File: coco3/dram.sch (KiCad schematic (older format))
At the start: 3 parts, among them CN4 Conn_01x12_Female, CN5 Conn_01x12_Female, CN6 Conn_01x12_Female

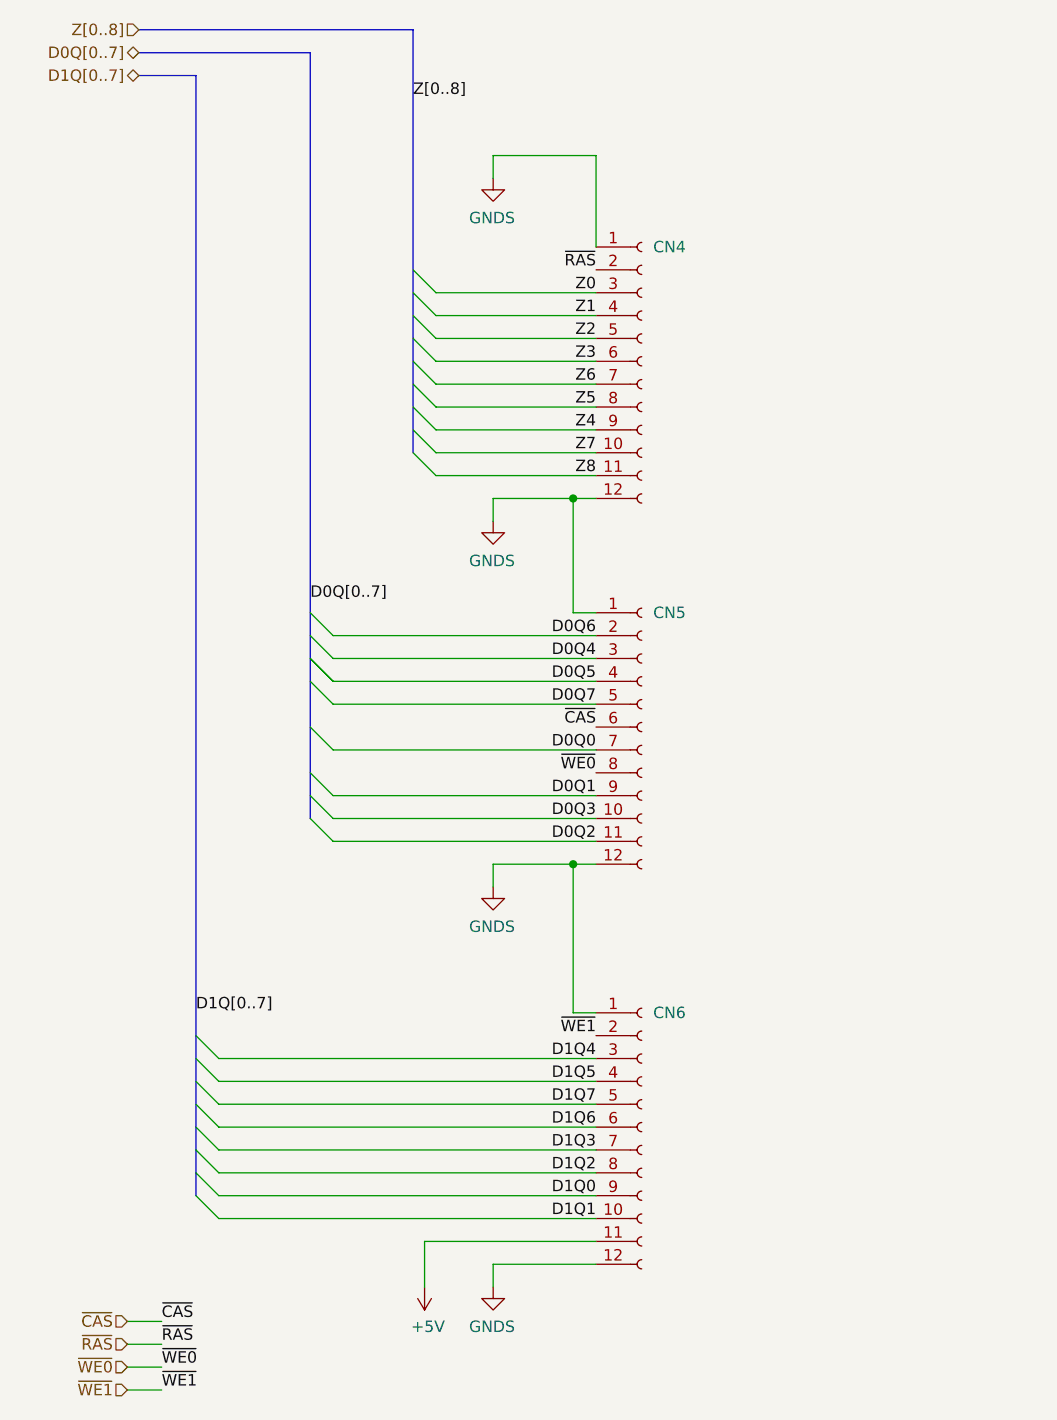
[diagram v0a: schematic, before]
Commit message: routed the board
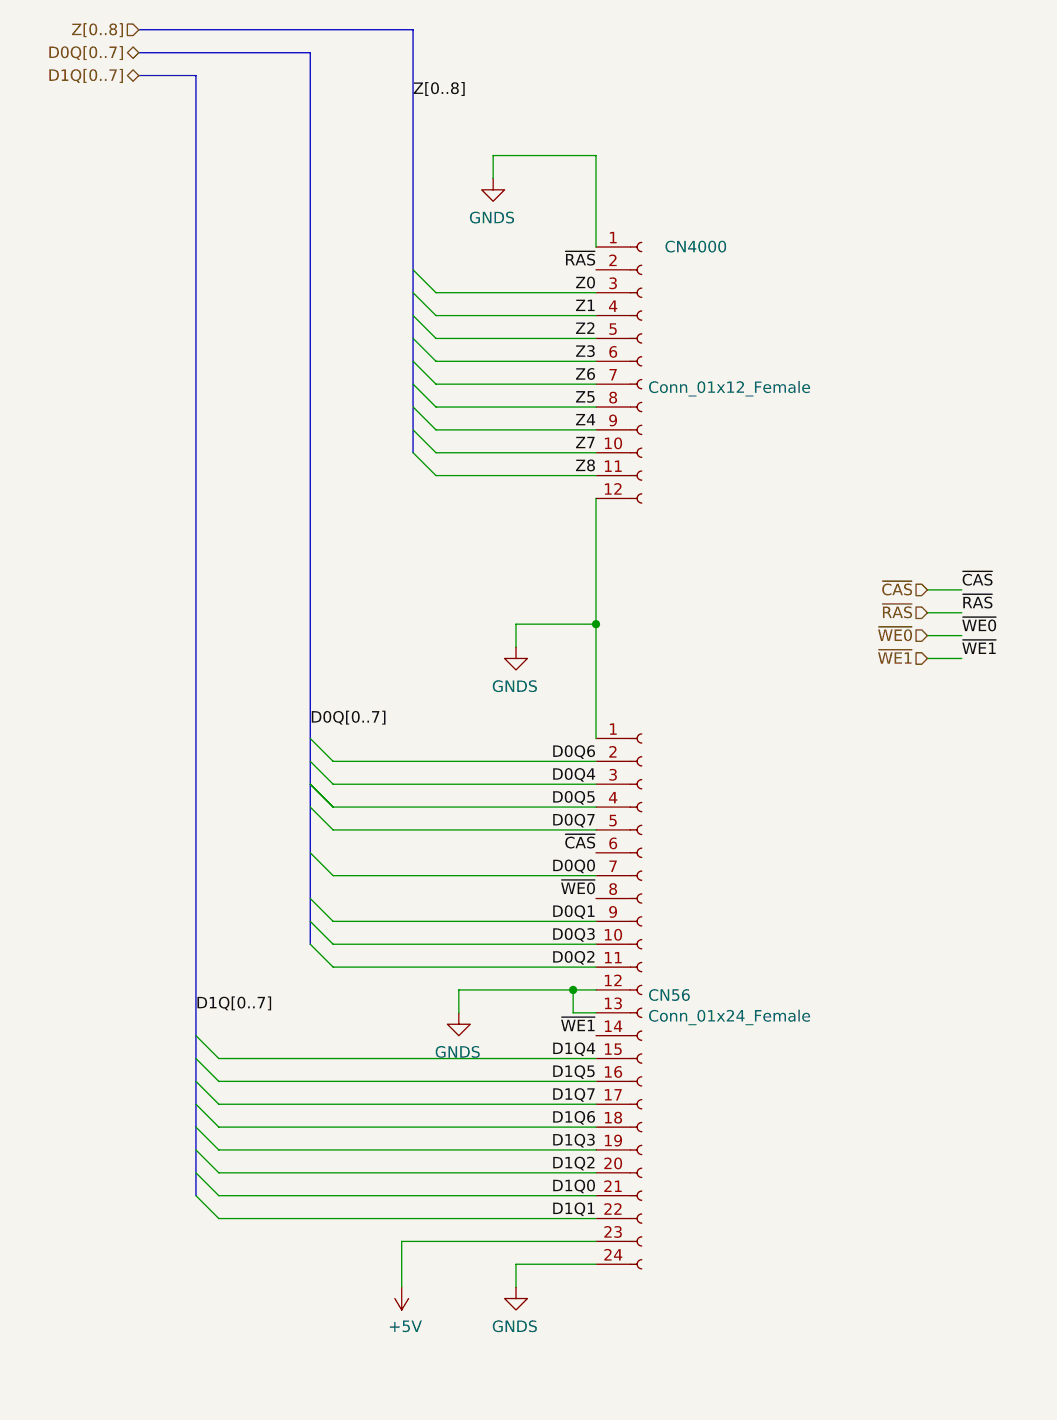
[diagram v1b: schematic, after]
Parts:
- removed CN4, CN5, CN6: Conn_01x12_Female, coco2:PinSocket_1x12_P2.54mm_for_memory_board_adapter, symbol Connector:Conn_01x12_Female
- added CN4000: Conn_01x12_Female, Connector_PinSocket_2.54mm:PinSocket_1x12_P2.54mm_Vertical, symbol Connector:Conn_01x12_Female
- added CN56: Conn_01x24_Female, Connector_PinSocket_2.54mm:PinSocket_1x24_P2.54mm_Vertical, symbol Connector:Conn_01x24_Female
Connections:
- net +5V: now also CN56.23 (Pin_23)
- net D0Q0: now also CN56.7 (Pin_7)
- net D0Q1: now also CN56.9 (Pin_9)
- net D0Q2: now also CN56.11 (Pin_11)
- net D0Q3: now also CN56.10 (Pin_10)
- net D0Q4: now also CN56.3 (Pin_3)
- net D0Q5: now also CN56.4 (Pin_4)
- net D0Q6: now also CN56.2 (Pin_2)
- net D0Q7: now also CN56.5 (Pin_5)
- net D1Q0: now also CN56.21 (Pin_21)
- net D1Q1: now also CN56.22 (Pin_22)
- net D1Q2: now also CN56.20 (Pin_20)
- net D1Q3: now also CN56.19 (Pin_19)
- net D1Q4: now also CN56.15 (Pin_15)
- net D1Q5: now also CN56.16 (Pin_16)
- net D1Q6: now also CN56.18 (Pin_18)
- net D1Q7: now also CN56.17 (Pin_17)
- net GNDS: now also CN4000.1 (Pin_1), CN4000.12 (Pin_12), CN56.1 (Pin_1), CN56.12 (Pin_12), CN56.13 (Pin_13), CN56.24 (Pin_24)
- net Z0: now also CN4000.3 (Pin_3)
- net Z1: now also CN4000.4 (Pin_4)
- net Z2: now also CN4000.5 (Pin_5)
- net Z3: now also CN4000.6 (Pin_6)
- net Z4: now also CN4000.9 (Pin_9)
- net Z5: now also CN4000.8 (Pin_8)
- net Z6: now also CN4000.7 (Pin_7)
- net Z7: now also CN4000.10 (Pin_10)
- net Z8: now also CN4000.11 (Pin_11)
- net ~CAS: now also CN56.6 (Pin_6)
- net ~RAS: now also CN4000.2 (Pin_2)
- net ~WE0: now also CN56.8 (Pin_8)
- net ~WE1: now also CN56.14 (Pin_14)
